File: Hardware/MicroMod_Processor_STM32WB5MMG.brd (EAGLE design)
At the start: 160 x 100 mm, 0 parts

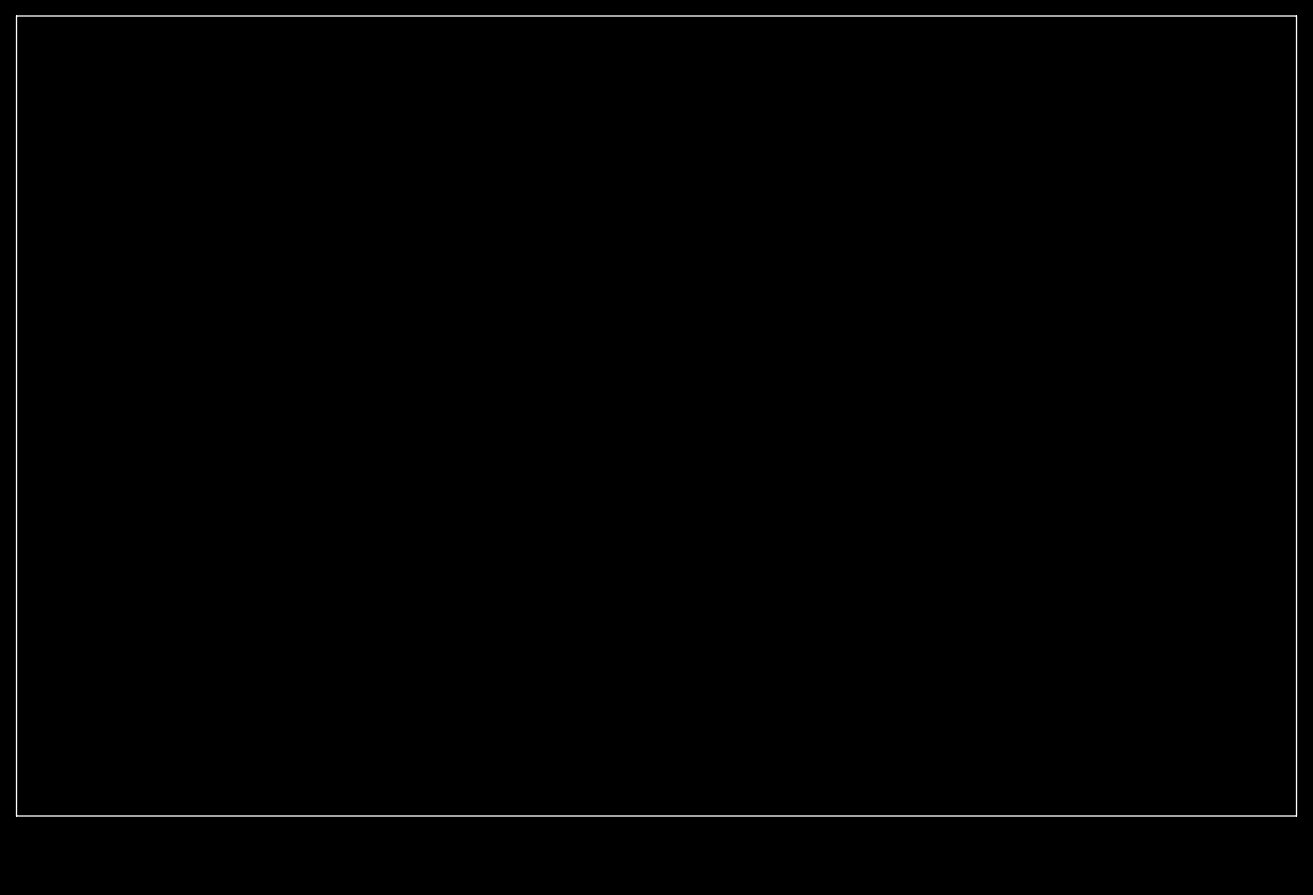
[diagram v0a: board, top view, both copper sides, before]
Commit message: Nearing layout completion.
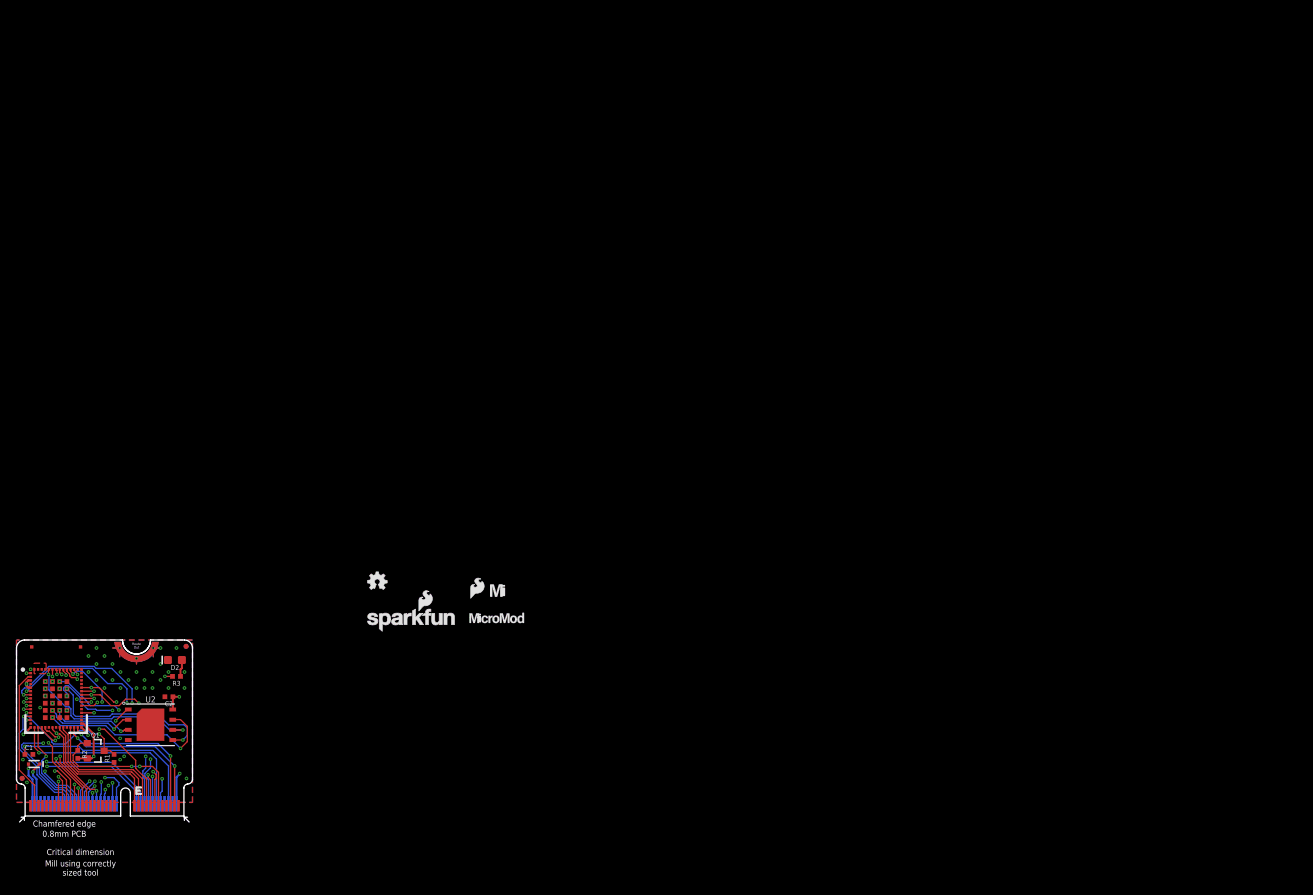
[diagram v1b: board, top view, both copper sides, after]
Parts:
- added C1, C2: 0.1uF, SparkFun-Capacitors:0402-TIGHT
- added D1: 120mA/40V/370mV, SparkFun-DiscreteSemi:SOD-523
- added D2: BLUE, SparkFun-LED:LED-0603
- added FD1, FD2, FD3, FD4: FIDUCIALUFIDUCIAL, SparkFun-Aesthetics:FIDUCIAL-MICRO
- added FRAME2: FRAME-LETTER, SparkFun-Aesthetics:CREATIVE_COMMONS
- added J1: MICROMOD-2222, SparkFun-MicroMod:M.2-CARD-E-22
- added LOGO1: FOUR_LAYER_WARNING, SparkFun-Aesthetics:FOUR_LAYER_WARNING
- added LOGO2: OSHW-LOGOMINI, SparkFun-Aesthetics:OSHW-LOGO-MINI
- added LOGO3: SFE_LOGO_NAME_FLAME.1_INCH, SparkFun-Aesthetics:SFE_LOGO_NAME_FLAME_.1
- added LOGO4: SPECIAL_INSTRUCTIONS-ORDERING, SparkFun-Aesthetics:ORDERING_INSTRUCTIONS
- added Q1: 20V/4.2A/52mΩ/1.4W, SparkFun-DiscreteSemi:SOT23-3
- added R1, R2: 100k, SparkFun-Resistors:0402-TIGHT
- added R3: 2.2k, SparkFun-Resistors:0402-TIGHT
- added U$1: (no value), SparkFun-MicroMod:MICROMOD_MI_LOGO_.35
- added U$2: (no value), SparkFun-MicroMod:MICROMOD_LOGO_.3
- added U$3: (no value), SparkFun-Aesthetics:SFE_LOGO_FLAME_.1
- added U1: STM32WB5MMG, stm32wb5mmg:SIP-LGA86
- added U2: W25QXX128MBIT-6X5, SparkFun-IC-Memory:WSON-8-6X5
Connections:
- new net !BOOT!: J1.11, Q1.1, R2.1
- new net !RESET!: C1.1, J1.6, U1.10
- new net 3.3V: C2.1, D1.A, J1.2, J1.74, Q1.2, R2.2, U1.17, U1.32, U1.4, U1.6, U2.8
- new net A0: J1.34, U1.8
- new net A1: J1.38, U1.7
- new net AUD_BCLK: J1.50, U1.50
- new net AUD_FSYNC: J1.52, U1.11
- new net AUD_I2S_IN: J1.54, U1.19
- new net AUD_I2S_OUT: J1.56, U1.38
- new net AUD_MCLK: J1.58, U1.14
- new net BATT_VIN: J1.49, U1.49
- new net BOOT0: Q1.3, R1.2, U1.13
- new net GND: C1.2, C2.2, D2.C, J1.1, J1.33, J1.36, J1.39, J1.45, J1.7, J1.75, J1.GND1, J1.GND2, J1.GND3, R1.1, U1.16, U1.31, U1.5, U1.57, U1.58, U1.59, U1.60, U1.84, U1.86, U2.4
- new net I2C1_INT: J1.16, U1.2
- new net I2C1_SCL: J1.14, U1.39
- new net I2C1_SDA: J1.12, U1.18
- new net I2C3_SCL: J1.53, U1.35
- new net I2C3_SDA: J1.51, U1.37
- new net LPUART_RX/DEV_TX: J1.20, U1.12
- new net LPUART_TX/DEV_RX: J1.22, U1.9
- new net N$1: D2.A, R3.1
- new net PA0/G5: J1.73, U1.3
- new net PC11/G1: J1.42, U1.23
- new net PC13/G2: J1.44, U1.40
- new net PD8/G3: J1.46, U1.75
- new net PE3/G4: J1.48, U1.72
- new net PE4/G0: J1.40, U1.42
- new net PH0/G7: J1.69, U1.61
- new net PH1/G6: J1.71, U1.62
- new net PWM0: J1.32, U1.63
- new net PWM1: J1.47, U1.76
- new net QSPI_!CS!: U1.70, U2.1
- new net QSPI_CLK: U1.56, U2.6
- new net QSPI_IO0: U1.73, U2.5
- new net QSPI_IO1: U1.80, U2.2
- new net QSPI_IO2: U1.81, U2.3
- new net QSPI_IO3: U1.67, U2.7
- new net SPI_!CS!: J1.55, U1.55
- new net SPI_PICO: J1.59, U1.52
- new net SPI_POCI: J1.61, U1.53
- new net SPI_SCK: J1.57, U1.54
- new net STAT: R3.2, U1.1
- new net SWDCK: J1.21, U1.26
- new net SWDIO: J1.23, U1.25
- new net TIM1_BKIN: J1.10, U1.41
- new net TIM1_ETR: J1.18, U1.79
- new net UART_CTS: J1.15, U1.20
- new net UART_RTS_DE: J1.13, U1.21
- new net UART_RX/DEV_TX: J1.19, U1.28
- new net UART_TX/DEV_RX: J1.17, U1.51
- new net USB_N: J1.5, U1.30
- new net USB_P: J1.3, U1.29
- new net V_BATT: D1.C, J1.72, U1.15
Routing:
- net A0: track 0.00 -> 33.5 mm, vias 0 -> 3
- net !RESET!: track 0.00 -> 31.8 mm, vias 0 -> 2
- net I2C1_INT: track 0.00 -> 31.5 mm, vias 0 -> 3
- net A1: track 0.00 -> 31.3 mm, vias 0 -> 3
- net TIM1_ETR: track 0.00 -> 27.6 mm, vias 0 -> 3
- net LPUART_TX/DEV_RX: track 0.00 -> 25.3 mm, vias 0 -> 2
- net TIM1_BKIN: track 0.00 -> 24.8 mm, vias 0 -> 2
- net PC13/G2: track 0.00 -> 24.7 mm, vias 0 -> 3
- net I2C1_SCL: track 0.00 -> 24.6 mm, vias 0 -> 2
- net LPUART_RX/DEV_TX: track 0.00 -> 24.1 mm, vias 0 -> 2
- net I2C1_SDA: track 0.00 -> 24.0 mm, vias 0 -> 1
- net AUD_I2S_OUT: track 0.00 -> 23.6 mm, vias 0 -> 2
- net QSPI_CLK: track 0.00 -> 23.4 mm, vias 0 -> 2
- net PD8/G3: track 0.00 -> 23.3 mm, vias 0 -> 4
- net QSPI_IO3: track 0.00 -> 22.9 mm, vias 0 -> 2
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- added copper zone on layer 15, net 3.3V
- added copper zone on layer 1, net GND
- added copper zone on layer 16, net GND
- added copper zone on layer 2, net GND
- added copper zone on layer 15, net GND1
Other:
- board size 160 x 100 mm -> 22 x 22 mm
- board text added: "Alex Brudner"
